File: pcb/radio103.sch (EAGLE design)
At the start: 124 parts, among them CON1 XT30PW-M, IC1 LM833D, IC10 78L05Z, IC2 7805TV, IC3 74ACT00D, IC4 MCP23S17SO, IC5 LM386M-1, IC6 LM1117MPX-3.3, IC7 4066D, IC8 LM833D, IC9 78L08Z, J1 PJ-324MH, J2 PJ-324MH, J3 PJ-324MH, SW1 EC12E_SW, SW2 EC12E_SW, T1 BC847, U1 FST3253

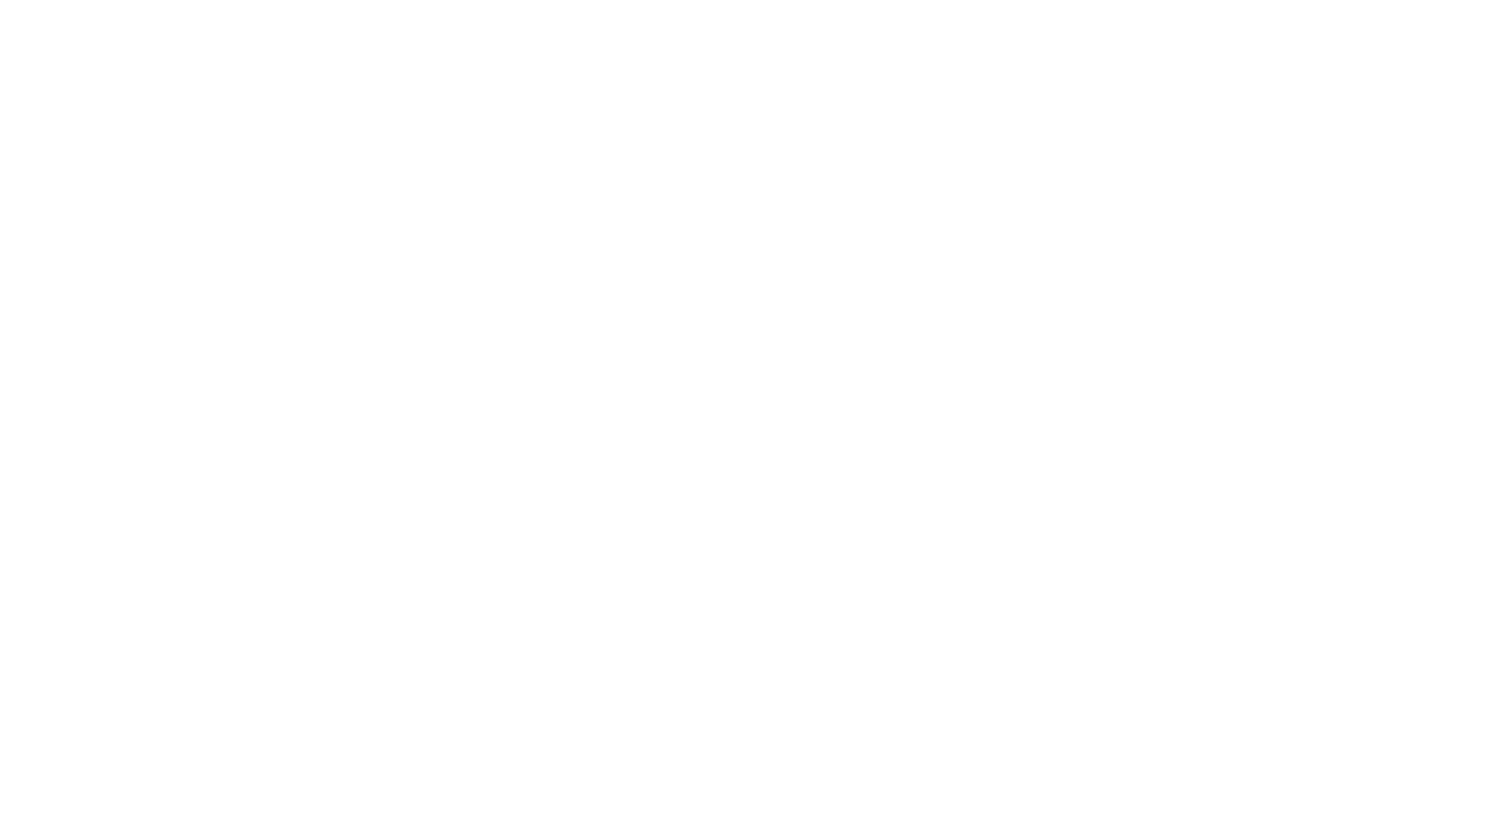
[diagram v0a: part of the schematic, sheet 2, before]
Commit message: gfx improved
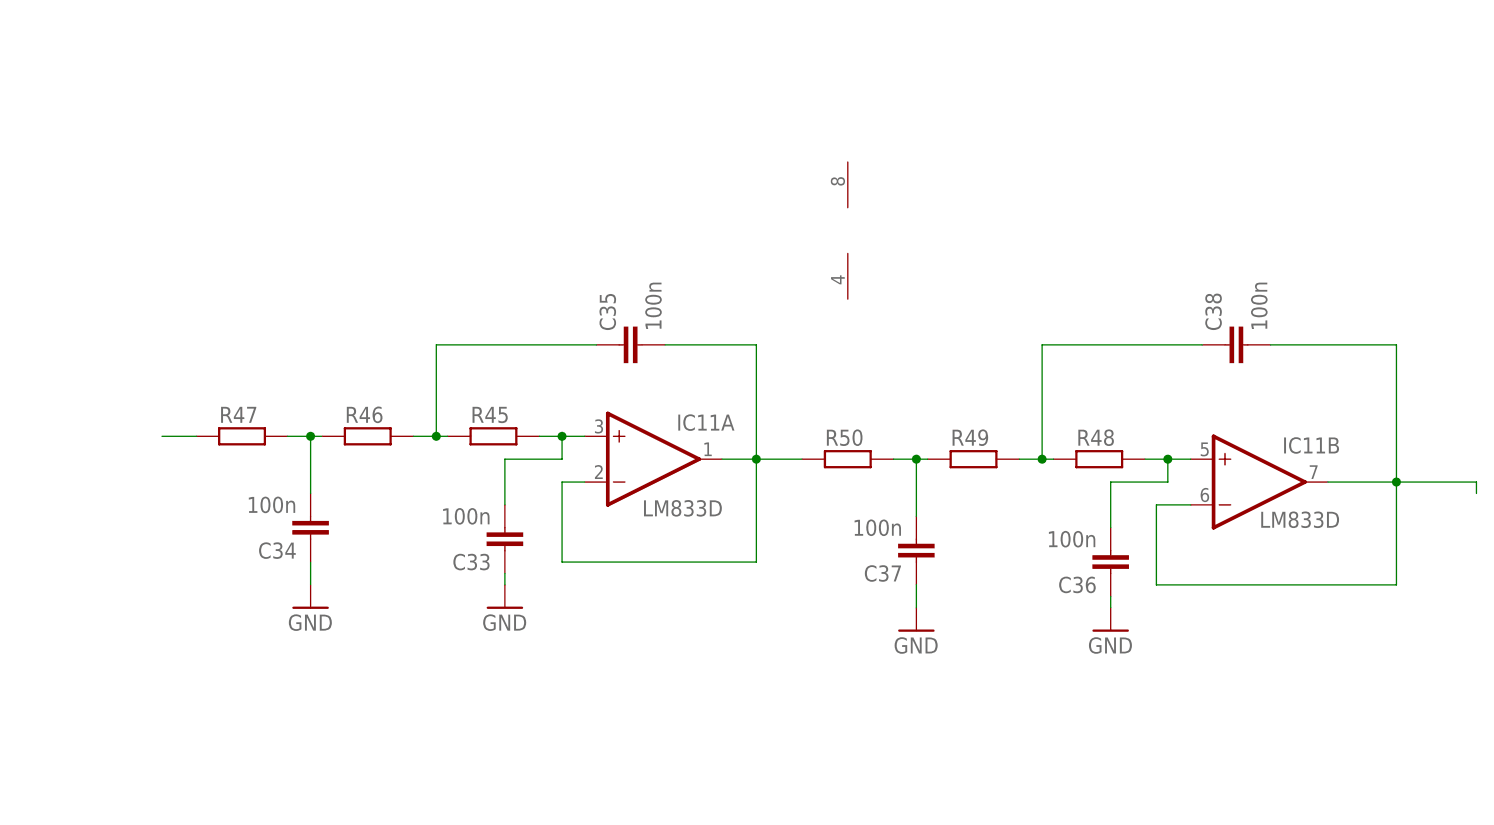
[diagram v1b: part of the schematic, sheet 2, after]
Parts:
- added C33, C34, C35, C36, C37, C38: 100n, rcl:C-EUC0805K
- added IC11: LM833D, linear:LM833D
- added R45, R46, R47, R48, R49, R50: (no value), rcl:R-EU_R0805
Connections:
- new net N$63: C33.2, IC11A.+IN, R45.2
- new net N$64: C35.1, R45.1, R46.2
- new net N$65: C35.2, IC11A.-IN, IC11A.OUT, R50.1
- new net N$66: C38.1, R48.1, R49.2
- new net N$67: C34.2, R46.1, R47.2
- new net N$68: R47.1
- new net N$69: C37.2, R49.1, R50.2
- new net N$71: C36.2, IC11B.+IN, R48.2
- new net N$73: C38.2, IC11B.-IN, IC11B.OUT
- net GND: now also C33.1, C34.1, C36.1, C37.1
